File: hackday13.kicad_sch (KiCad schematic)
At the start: 8 parts, among them J1 TT-output, J2 TT-input, SW1 Reset button, SW2 SW_DIP_x02, U1 RaspberryPi_Pico

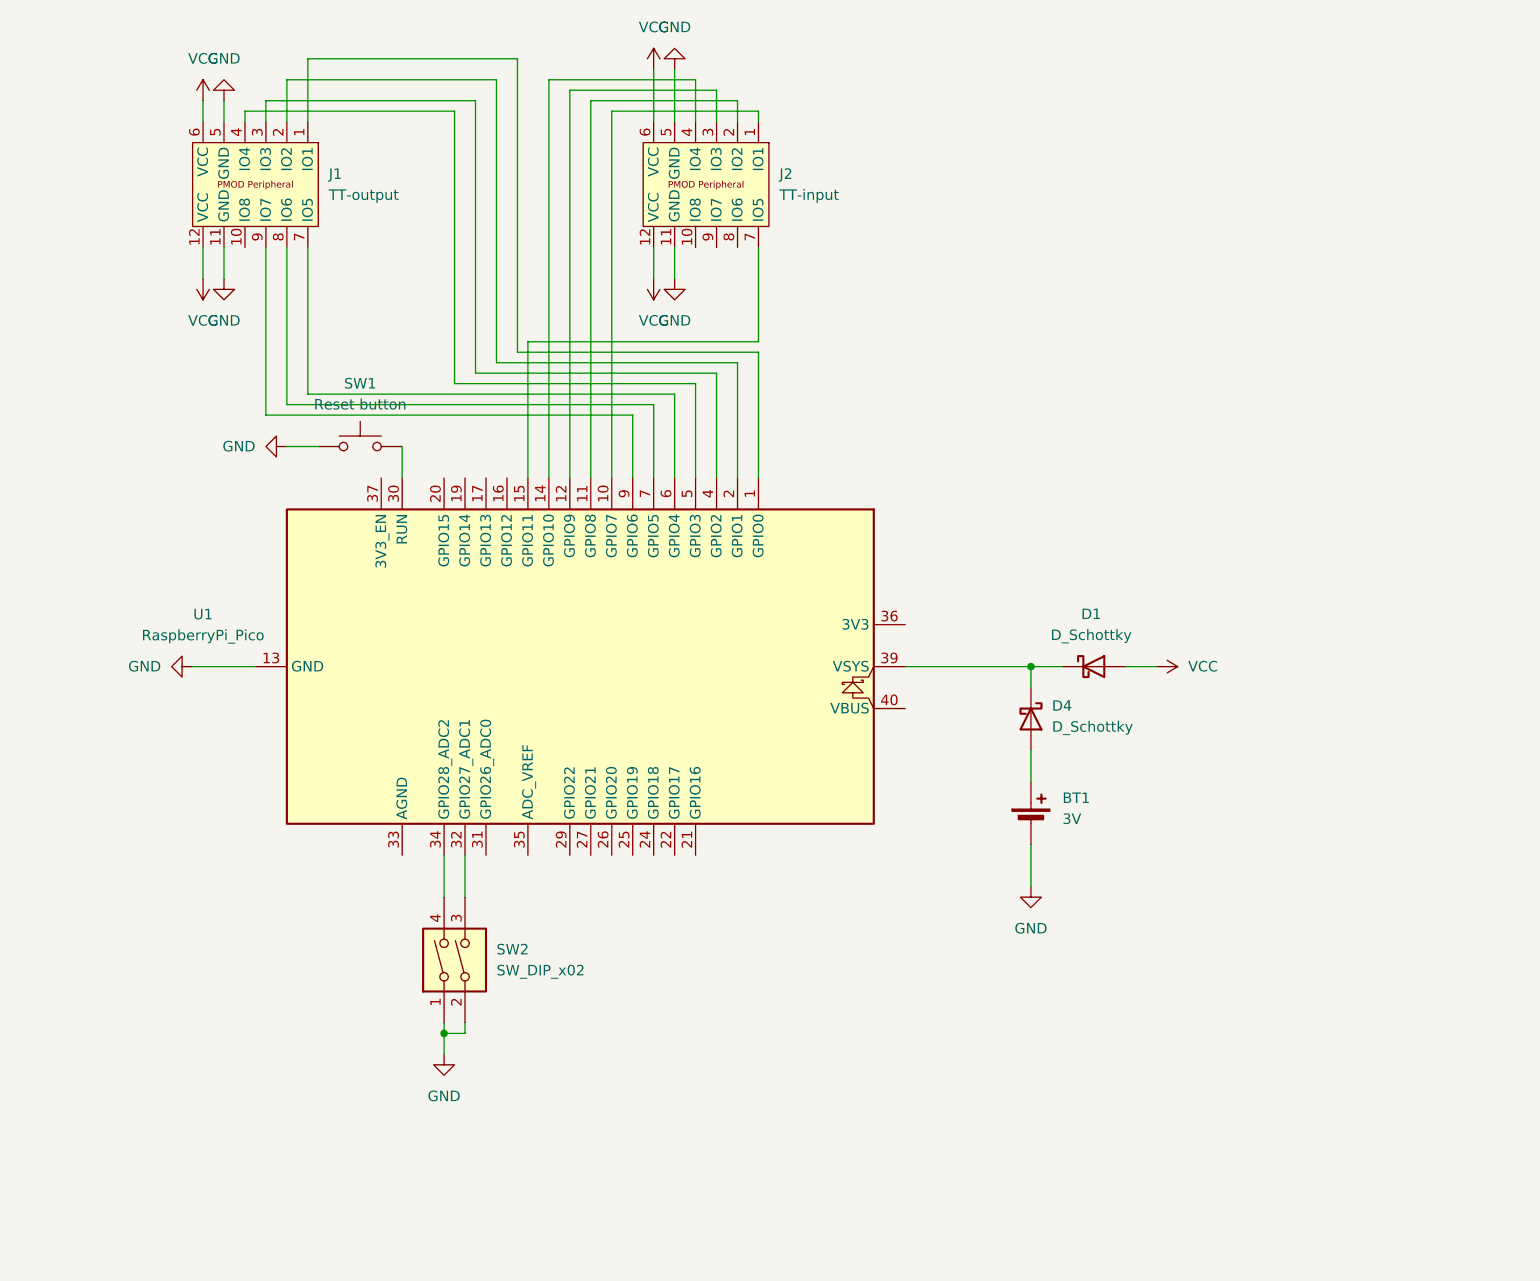
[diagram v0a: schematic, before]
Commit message: Add LED dot matrix schematic
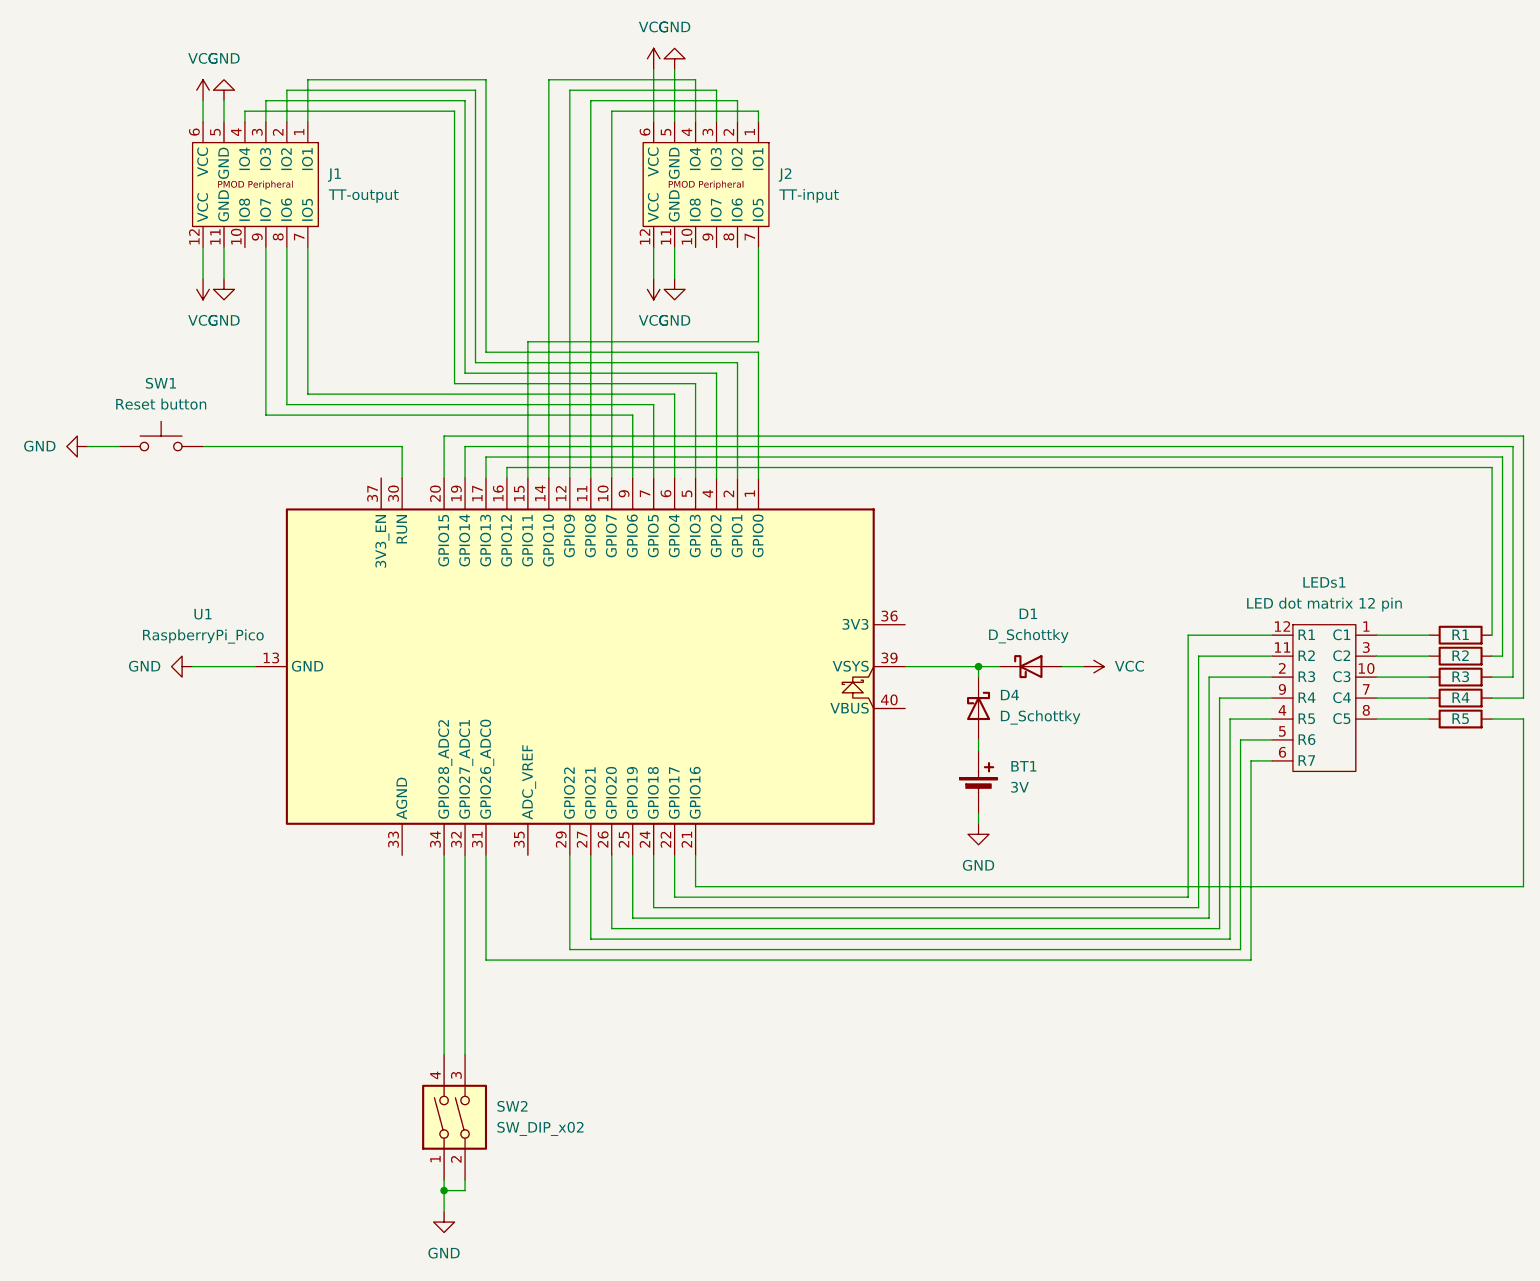
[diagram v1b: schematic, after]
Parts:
- added LEDs1: LED dot matrix 12 pin, symbol custom_components_led_pcb:TA07-11SEKWA
- added R1, R2, R3, R4, R5: R, symbol Device:R
- BT1: footprint Battery:BatteryHolder_Keystone_105_1x2430 -> Battery:BatteryHolder_Keystone_3002_1x2032
- SW2: footprint (none) -> Button_Switch_THT:SW_DIP_SPSTx02_Slide_9.78x7.26mm_W7.62mm_P2.54mm
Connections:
- net at U1.16 (GPIO12): now also R1.2
- net at U1.17 (GPIO13): now also R2.2
- net at U1.19 (GPIO14): now also R3.2
- net at U1.20 (GPIO15): now also R4.2
- net at U1.21 (GPIO16): now also R5.2
- net at U1.22 (GPIO17): now also LEDs1.12 (R1)
- net at U1.24 (GPIO18): now also LEDs1.11 (R2)
- net at U1.25 (GPIO19): now also LEDs1.2 (R3)
- net at U1.26 (GPIO20): now also LEDs1.9 (R4)
- net at U1.27 (GPIO21): now also LEDs1.4 (R5)
- net at U1.29 (GPIO22): now also LEDs1.5 (R6)
- net at U1.31 (GPIO26_ADC0): now also LEDs1.6 (R7)
- new net: LEDs1.3 (C2), R2.1
- new net: LEDs1.10 (C3), R3.1
- new net: LEDs1.1 (C1), R1.1
- new net: LEDs1.7 (C4), R4.1
- new net: LEDs1.8 (C5), R5.1
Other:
- moved on the sheet: BT1, D1, D4, SW1, SW2
